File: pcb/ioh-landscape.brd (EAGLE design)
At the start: 80 x 41.9 mm, 35 parts

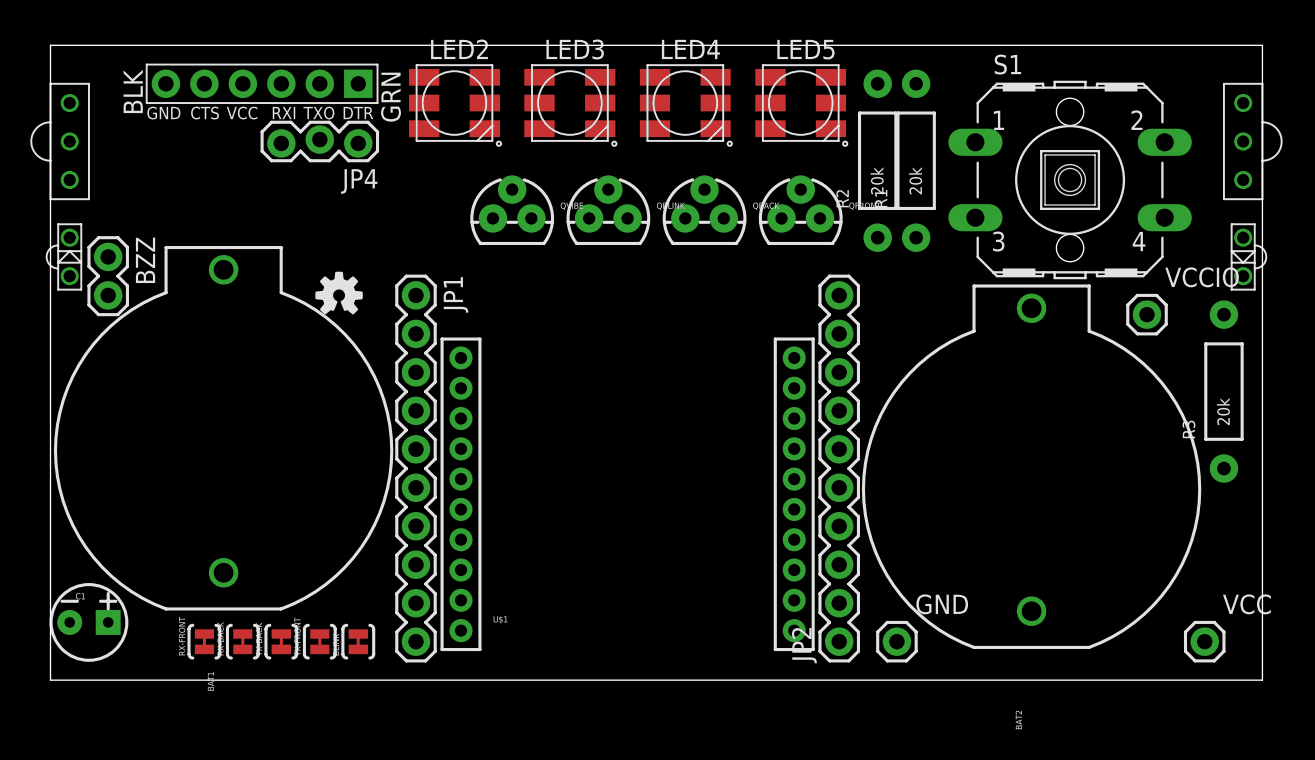
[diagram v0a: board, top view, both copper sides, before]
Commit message: routed
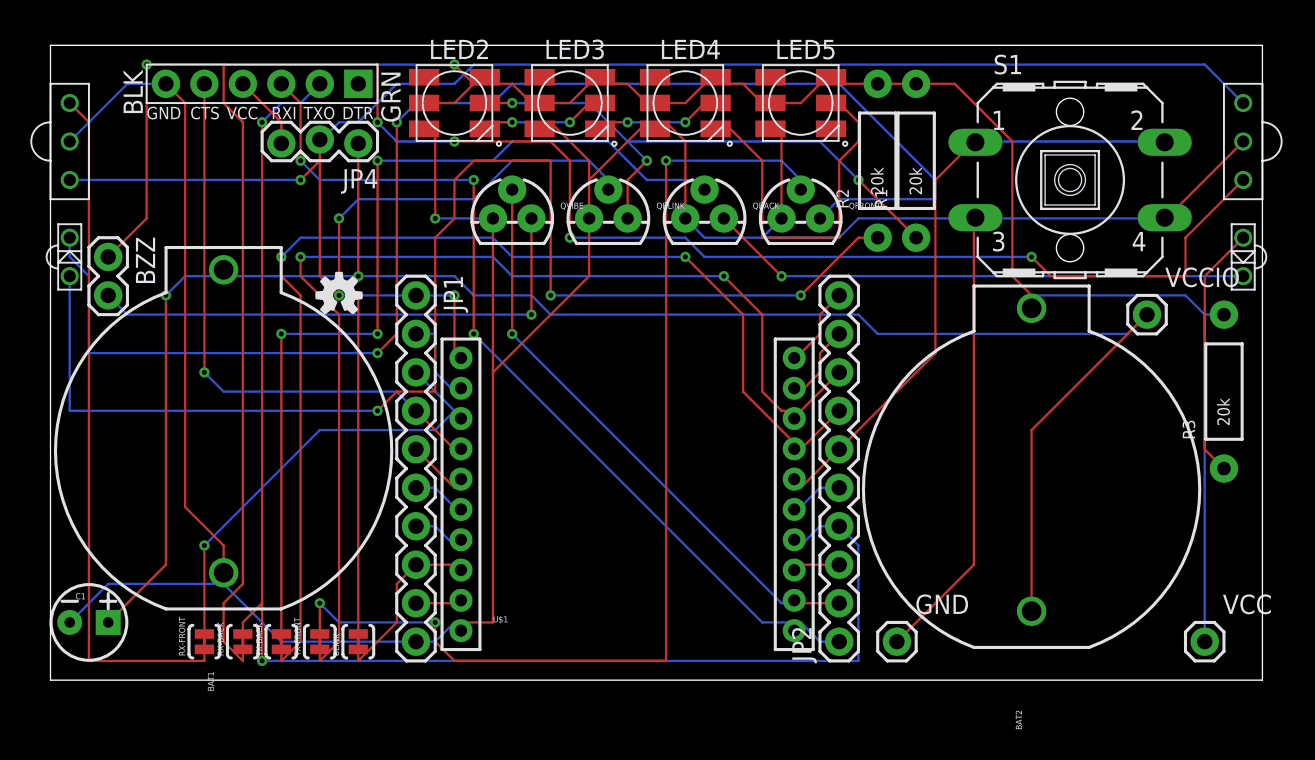
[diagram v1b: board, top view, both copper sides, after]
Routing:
- net GND: track 0.00 -> 226.7 mm, vias 0 -> 1
- net VCC: track 0.00 -> 128.2 mm, vias 0 -> 2
- net N$15: track 0.00 -> 124.1 mm, vias 0 -> 4
- net N$14: track 0.00 -> 122.6 mm, vias 0 -> 2
- net VCCIO: track 0.00 -> 104.1 mm, vias 0 -> 3
- net RXBACK: track 0.00 -> 95.4 mm, vias 0 -> 2
- net N$11: track 0.00 -> 91.6 mm, vias 0 -> 2
- net N$4: track 0.00 -> 87.0 mm, vias 0 -> 3
- net TXBACK: track 0.00 -> 76.1 mm, vias 0 -> 2
- net TXFRONT: track 0.00 -> 73.5 mm, vias 0 -> 2
- net N$20: track 0.00 -> 70.3 mm, vias 0 -> 3
- net N$21: track 0.00 -> 61.4 mm, vias 0 -> 3
- net TX0: track 0.00 -> 61.0 mm, vias 0 -> 3
- net N$6: track 0.00 -> 48.5 mm, vias 0 -> 1
- net N$17: track 0.00 -> 45.7 mm
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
